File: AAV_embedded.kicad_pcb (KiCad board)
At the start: 4 copper layers, 165.8 x 114.2 mm, 51 parts, among them J1 JTAG_SWD_CONN, J10 DRV_HIGH_C2, J11 DRV_LOW_C2, J12 DRV_HIGH_C3, J13 DRV_LOW_C3, J14 DRV_LOW_C1, J2 12v in, J3 USB_C_Receptacle_USB2.0_14P, J5 THR_EN_JMP, J6 GPIO_INTERNAL_PINS, J7 GPIO_EXT_PINS, J8 Conn_01x03_Pin, J9 DRV_HIGH_C1, SW1 DAC_ADDR, SW2 IO_EXT_ADDR, SW3 SW_DIP_x03, SW4 5v_USB_EN, SW5 DAC_EN, U1 DAC101C081CIMK, U2 PCA9555D, U3 LD1117S50TR_SOT223, U4 LD1117S33TR_SOT223, U5 FXMA108

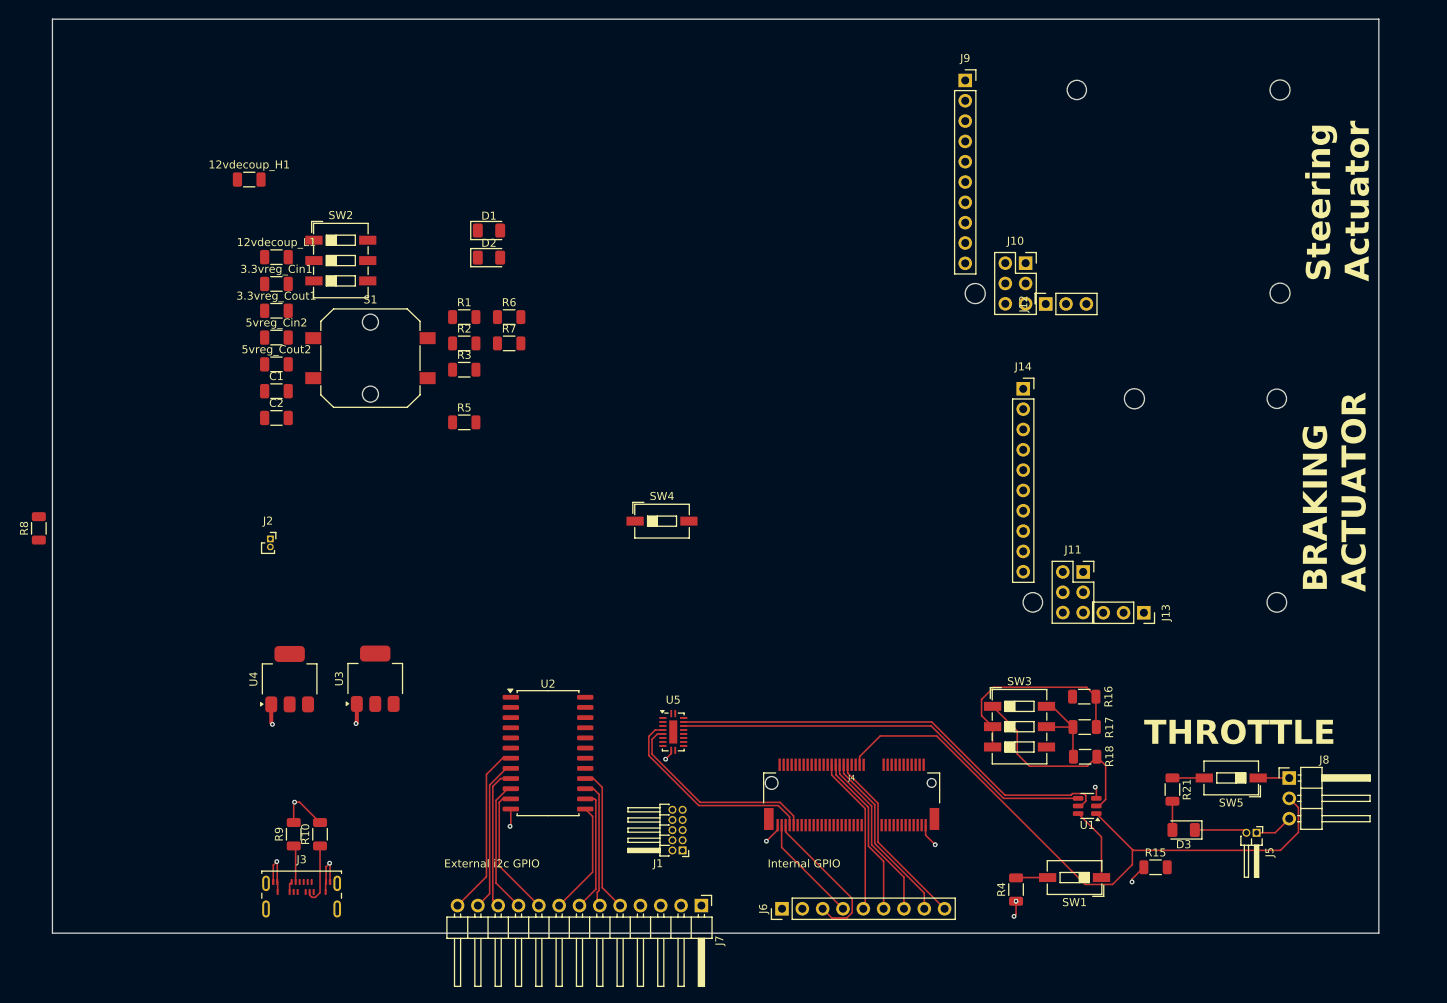
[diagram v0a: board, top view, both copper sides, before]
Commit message: board layout v1
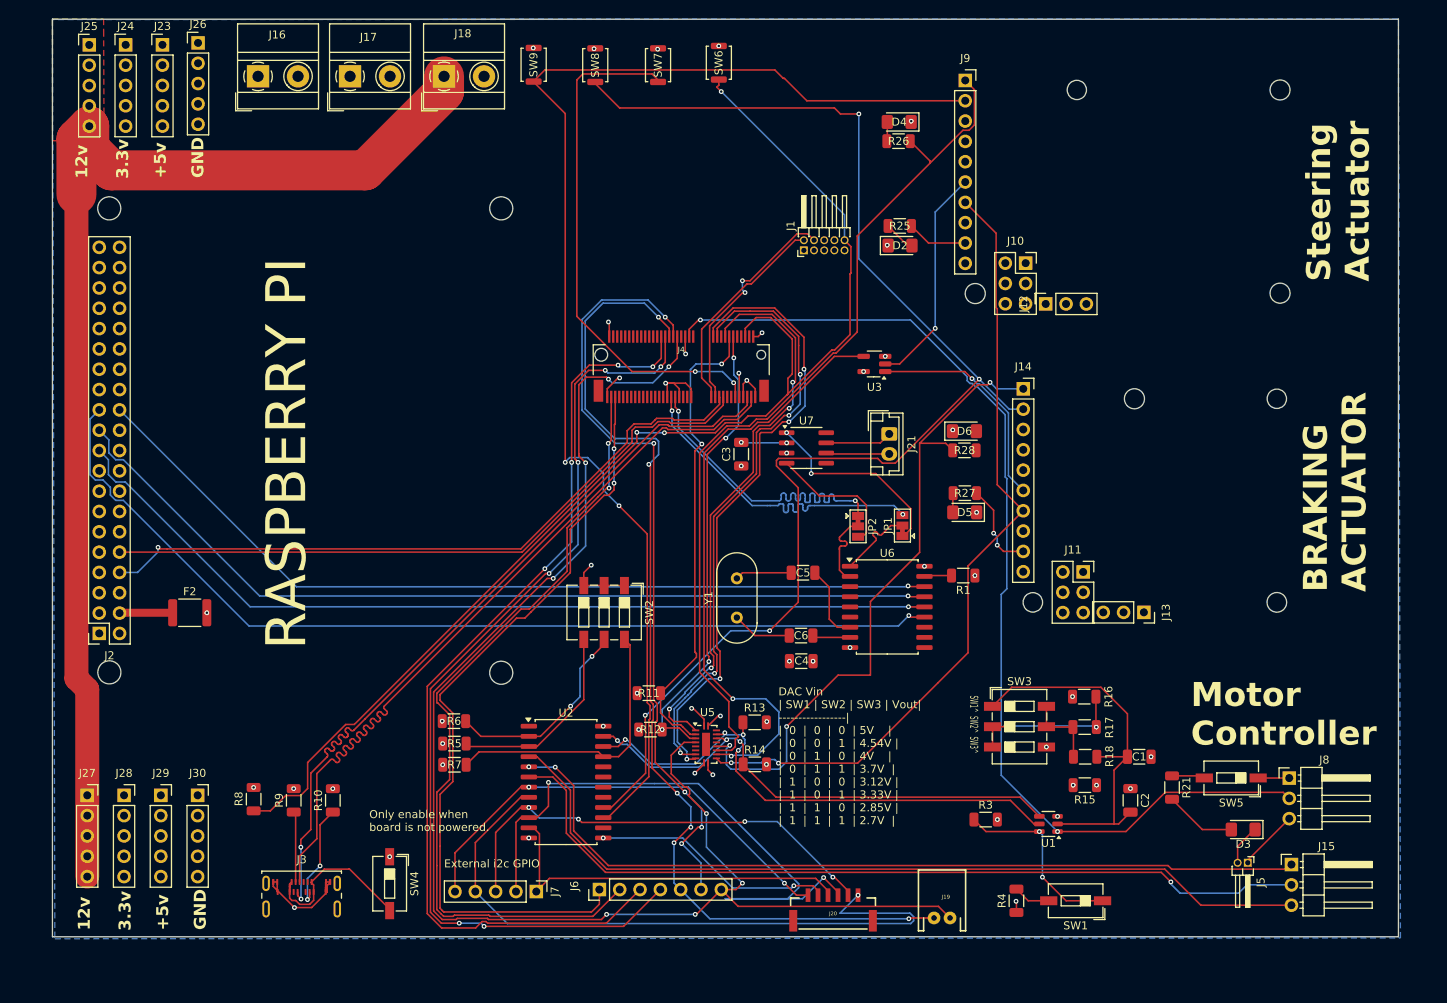
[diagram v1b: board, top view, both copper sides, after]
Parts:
- removed 12vdecoup_H1: 0.1uF, Capacitor_SMD:C_1206_3216Metric
- removed 12vdecoup_L1: 100uF, Capacitor_SMD:C_1206_3216Metric
- removed 3.3vreg_Cin1, 5vreg_Cin2: 100nF, Capacitor_SMD:C_1206_3216Metric
- removed 3.3vreg_Cout1, 5vreg_Cout2: 10uF, Capacitor_SMD:C_1206_3216Metric
- removed D1: D_Schottky_low_forward, Diode_SMD:D_1206_3216Metric
- removed R2: 2k, Resistor_SMD:R_1206_3216Metric
- removed S1: GPTS203211B, Button_Switch_SMD:SW_Push_1P1T_NO_CK_PTS125Sx43PSMTR
- removed U4: LD1117S33TR_SOT223, Package_TO_SOT_SMD:SOT-223-3_TabPin2
- added C3: 0.1uF, Capacitor_SMD:C_1206_3216Metric, F.Cu at (134.1, 97.5)
- added C4: 0.1uF, Capacitor_SMD:C_1206_3216Metric, F.Cu at (141.6, 123.4)
- added C5: 22pF, Capacitor_SMD:C_1206_3216Metric, F.Cu at (141.8, 112.3)
- added C6: 22pF, Capacitor_SMD:C_1206_3216Metric, F.Cu at (141.5, 120.2)
- added D4: LED, LED_SMD:LED_1206_3216Metric_Pad1.42x1.75mm_HandSolder, F.Cu at (153.8, 56.0)
- added D5: LED, LED_SMD:LED_1206_3216Metric_Pad1.42x1.75mm_HandSolder, F.Cu at (162.0, 104.8)
- added D6: LED, LED_SMD:LED_1206_3216Metric_Pad1.42x1.75mm_HandSolder, F.Cu at (161.9, 94.7)
- added F2: Polyfuse_3A_15V, Fuse:Fuse_1812_4532Metric, F.Cu at (65.1, 117.3)
- added J15: Brake/FwRev, Connector_PinHeader_2.54mm:PinHeader_1x03_P2.54mm_Horizontal, F.Cu at (202.8, 148.8)
- added J16: 5v_in, TerminalBlock_MetzConnect:TerminalBlock_MetzConnect_Type011_RT05502HBWC_1x02_P5.00mm_Horizontal, F.Cu at (73.7, 50.3)
- added J17: 3.3v_in, TerminalBlock_MetzConnect:TerminalBlock_MetzConnect_Type011_RT05502HBWC_1x02_P5.00mm_Horizontal, F.Cu at (85.2, 50.3)
- added J18: 12v_in, TerminalBlock_MetzConnect:TerminalBlock_MetzConnect_Type011_RT05502HBWC_1x02_P5.00mm_Horizontal, F.Cu at (96.9, 50.3)
- added J19: ~, SparkFun-Connectors:JST-2-PTH, F.Cu at (159.2, 155.5)
- added J20: ~, SparkFun-Connectors:JST-6-SMD-1.25MM-LOCKING, F.Cu at (145.5, 155.9)
- added J21: CAN, Connector_JST:JST_EH_B2B-EH-A_1x02_P2.50mm_Vertical, F.Cu at (152.6, 95.0)
- added J23: 5v_rail, Connector_PinHeader_2.54mm:PinHeader_1x05_P2.54mm_Vertical, F.Cu at (61.7, 46.4)
- added J24: 3.3v_rail, Connector_PinHeader_2.54mm:PinHeader_1x05_P2.54mm_Vertical, F.Cu at (57.1, 46.4)
- added J25: 12v_rail, Connector_PinHeader_2.54mm:PinHeader_1x05_P2.54mm_Vertical, F.Cu at (52.5, 46.4)
- added J26: GND_rail, Connector_PinHeader_2.54mm:PinHeader_1x05_P2.54mm_Vertical, F.Cu at (66.2, 46.1)
- added J27: 12v_rail_f, Connector_PinSocket_2.54mm:PinSocket_1x05_P2.54mm_Vertical, F.Cu at (52.3, 140.2)
- added J28: 3.3v_rail_f, Connector_PinSocket_2.54mm:PinSocket_1x05_P2.54mm_Vertical, F.Cu at (56.9, 140.2)
- added J29: 5v_rail_f, Connector_PinSocket_2.54mm:PinSocket_1x05_P2.54mm_Vertical, F.Cu at (61.5, 140.2)
- added J30: GND_rail_f, Connector_PinSocket_2.54mm:PinSocket_1x05_P2.54mm_Vertical, F.Cu at (66.1, 140.2)
- added JP1: CAN_TXD_SEL, Jumper:SolderJumper-3_P1.3mm_Bridged12_Pad1.0x1.5mm, F.Cu at (154.2, 106.5)
- added JP2: CAN_RXD_SEL, Jumper:SolderJumper-3_P1.3mm_Bridged12_Pad1.0x1.5mm, F.Cu at (148.7, 106.5)
- added R11: 2k, Resistor_SMD:R_1206_3216Metric, F.Cu at (122.5, 127.4)
- added R12: 2k, Resistor_SMD:R_1206_3216Metric, F.Cu at (122.7, 131.9)
- added R13: 2k, Resistor_SMD:R_1206_3216Metric, F.Cu at (135.7, 131.1)
- added R14: 2k, Resistor_SMD:R_1206_3216Metric, F.Cu at (135.8, 136.3)
- added R25: 10k, Resistor_SMD:R_1206_3216Metric, F.Cu at (153.9, 69.0)
- added R26: 10k, Resistor_SMD:R_1206_3216Metric, F.Cu at (153.7, 58.4)
- added R27: 10k, Resistor_SMD:R_1206_3216Metric, F.Cu at (162.0, 102.4)
- added R28: 10k, Resistor_SMD:R_1206_3216Metric, F.Cu at (161.9, 97.0)
- added SW6: ~{RESET_uMOD}, Button_Switch_SMD:SW_Push_SPST_NO_Alps_SKRK, F.Cu at (131.2, 48.6)
- added SW7: ~{BOOT_uMOD}, Button_Switch_SMD:SW_Push_SPST_NO_Alps_SKRK, F.Cu at (123.7, 48.9)
- added SW8: ~{RESET_BRK}, Button_Switch_SMD:SW_Push_SPST_NO_Alps_SKRK, F.Cu at (115.8, 48.9)
- added SW9: ~{RESET_STR}, Button_Switch_SMD:SW_Push_SPST_NO_Alps_SKRK, F.Cu at (108.1, 48.9)
- added U6: MCP2515-xSO, Package_SO:SOIC-18W_7.5x11.6mm_P1.27mm, F.Cu at (152.3, 116.6)
- added U7: SN65HVD230, Package_SO:SOIC-8_3.9x4.9mm_P1.27mm, F.Cu at (142.2, 96.8)
- added Y1: 16MHz, Crystal:Crystal_HC18-U_Vertical, F.Cu at (133.5, 118.0)
- D2: value D_TVS -> LED; footprint Diode_SMD:D_1206_3216Metric -> LED_SMD:LED_1206_3216Metric_Pad1.42x1.75mm_HandSolder
- D3: footprint LED_SMD:LED_1206_3216Metric -> LED_SMD:LED_1206_3216Metric_Pad1.42x1.75mm_HandSolder
- J2: value 12v in -> Raspberry_Pi_4; footprint Connector_PinSocket_1.00mm:PinSocket_1x02_P1.00mm_Vertical -> Connector_PinSocket_2.54mm:PinSocket_2x20_P2.54mm_Vertical
- J6: value GPIO_INTERNAL_PINS -> Conn_01x07; footprint Connector_PinHeader_2.54mm:PinHeader_1x09_P2.54mm_Vertical -> Connector_PinHeader_2.54mm:PinHeader_1x07_P2.54mm_Vertical
- J7: value GPIO_EXT_PINS -> Conn_01x05; footprint Connector_PinHeader_2.54mm:PinHeader_1x13_P2.54mm_Horizontal -> Connector_PinHeader_2.54mm:PinHeader_1x05_P2.54mm_Vertical
- J8: value Conn_01x03_Pin -> Throttle Connector
- R1: value 2k -> 10k
- SW5: value DAC_EN -> THR_EN
- U3: value LD1117S50TR_SOT223 -> 74AHC1G08; footprint Package_TO_SOT_SMD:SOT-223-3_TabPin2 -> Package_TO_SOT_SMD:SOT-23-5_HandSoldering
- moved C1 117.1 mm to (183.8, 135.3), turned to 180 degrees
- moved C2 117.0 mm to (182.7, 140.8), turned to -90 degrees
- moved R3 86.1 mm to (164.6, 143.2)
- moved J1 76.5 mm to (141.9, 72.0), turned to 90 degrees
- moved U3 73.8 mm to (150.7, 86.2), turned to 180 degrees
- moved R1 70.2 mm to (161.8, 112.7), turned to 180 degrees
- moved J4 57.6 mm to (126.5, 85.1)
- moved SW4 56.7 mm to (90.1, 151.2), turned to -90 degrees
- moved SW2 54.9 mm to (116.9, 117.3), turned to -90 degrees
- moved R7 53.1 mm to (98.2, 136.3)
- moved D2 51.4 mm to (153.9, 71.5)
- moved R6 51.0 mm to (98.1, 130.9)
- moved R8 43.2 mm to (73.1, 140.7), turned to -90 degrees
- moved R5 40.2 mm to (98.2, 133.7)
- moved J2 24.4 mm to (53.8, 119.9), turned to 180 degrees
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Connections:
- net RST renamed ~{RESET_uMOD}
- D2 pad 1: Net-(D1-A) -> GND
- D2 pad 2: GND -> Net-(D2-A)
- J14 pad 1: ERR_LOW -> ERR_BRK
- J14 pad 2: ~{RST_LOW} -> ~{RST_BRK}
- J14 pad 6: TX_LOW_5v -> TX_BRK_5v
- J14 pad 7: RX_LOW_5v -> RX_DRV_5v
- J14 pad 9: 5v_reg_LOW -> 5v_reg_BRK
- J2 pad 1: GND -> Net-(J2-3V3-Pad1)
- J2 pad 2: Net-(D1-A) -> Net-(F2-Pad1)
- J4 pad 11: unconnected-(J4-~{BOOT}-Pad11) -> ~{BOOT_uMOD}
- J4 pad 17: unconnected-(J4-TX1-Pad17) -> uMod_TX1
- J4 pad 19: unconnected-(J4-RX1-Pad19) -> uMod_RX1
- J4 pad 2: Net-(J4-3.3V-Pad2) -> +3.3V
- J4 pad 20: unconnected-(J4-RX2-Pad20) -> TX_DRV_L
- J4 pad 22: unconnected-(J4-TX2-Pad22) -> RX_DRV_L
- J4 pad 40: GPIO_INTERNAL_0 -> ~{E-STOP}
- J4 pad 41: unconnected-(J4-CAN-RX-Pad41) -> CAN_RXD
- J4 pad 42: GPIO_INTERNAL_1 -> ERR_L
- J4 pad 43: unconnected-(J4-CAN-TX-Pad43) -> CAN_TXD
- J4 pad 44: GPIO_INTERNAL_2 -> ~{E-STOP-TRIG}
- J4 pad 51: SDA _MCTRL_L -> unconnected-(J4-I2C_SDA1-Pad51)
- J4 pad 53: SCL_MCTRL_L -> unconnected-(J4-I2C_SCL1-Pad53)
- J4 pad 67: ERR_HIGH_L -> GPIO_INTERNAL_8
- J4 pad 69: ERR_LOW_L -> GPIO_INTERNAL_7
- J4 pad 74: Net-(J4-3.3V-Pad2) -> +3.3V
- J4 pad 9: unconnected-(J4-USB_VIN-Pad9) -> +5V
- J6 pad 1: GPIO_INTERNAL_8 -> GPIO_INTERNAL_6
- J6 pad 2: GPIO_INTERNAL_7 -> GPIO_INTERNAL_5
- J6 pad 3: GPIO_INTERNAL_6 -> GPIO_INTERNAL_4
- J6 pad 4: GPIO_INTERNAL_5 -> GPIO_INTERNAL_3
- J6 pad 5: GPIO_INTERNAL_4 -> ~{E-STOP-TRIG}
- J6 pad 6: GPIO_INTERNAL_3 -> ERR_L
- J6 pad 7: GPIO_INTERNAL_2 -> ~{E-STOP}
- J7 pad 1: GPIO_EXT_12 -> GPIO_EXT_4
- J7 pad 2: GPIO_EXT_11 -> GPIO_EXT_3
- J7 pad 3: GPIO_EXT_10 -> GPIO_EXT_2
- J7 pad 4: GPIO_EXT_9 -> GPIO_EXT_1
- J7 pad 5: GPIO_EXT_8 -> GPIO_EXT_0
- J9 pad 1: ERR_HIGH -> ERR_STR
- J9 pad 2: ~{RST_HIGH} -> ~{RST_STR}
- J9 pad 6: TX_HIGH_5v -> TX_STR_5v
- J9 pad 7: RX_HIGH_5v -> RX_DRV_5v
- J9 pad 9: 5v_reg_HIGH -> 5v_reg_STR
- R1 pad 1: +5V -> GND
- R1 pad 2: SCL_1_H -> Net-(U6-~{RESET})
- U2 pad 15: GPIO_EXT_7 -> ~{RST_STR}
- U2 pad 16: GPIO_EXT_8 -> ~{RST_BRK}
- U3 pad 1: GND -> TX_BRK_5v
- U3 pad 2: +5V -> TX_STR_5v
- U3 pad 3: +12v -> GND
- U5 pad 12: unconnected-(U5-B7-Pad12) -> RX_DRV_5v
- U5 pad 13: unconnected-(U5-B6-Pad13) -> TX_DRV_5v
- U5 pad 14: unconnected-(U5-B5-Pad14) -> ERR_STR
- U5 pad 15: ERR_HIGH -> ERR_BRK
- U5 pad 16: ERR_LOW -> ~{ERR}
- U5 pad 5: ERR_LOW_L -> ~{E-STOP}
- U5 pad 6: ERR_HIGH_L -> ERR_BRK_L
- U5 pad 7: unconnected-(U5-A5-Pad7) -> ERR_STR_L
- U5 pad 8: unconnected-(U5-A6-Pad8) -> TX_DRV_L
- U5 pad 9: unconnected-(U5-A7-Pad9) -> RX_DRV_L
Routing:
- net ~{E-STOP}: track 0.00 -> 186.2 mm, vias 0 -> 8
- net ~{RST_BRK}: track 0.00 -> 169.4 mm, vias 0 -> 4
- net ~{RST_STR}: track 0.00 -> 159.5 mm, vias 0 -> 2
- net ~{RESET_uMOD}: track 0.00 -> 156.7 mm, vias 0 -> 3
- net +12V: track 0.00 -> 150.5 mm
- net ~{E-STOP-TRIG}: track 0.00 -> 129.0 mm, vias 0 -> 6
- net CAN_SCK: track 0.00 -> 121.9 mm, vias 0 -> 1
- net CAN_MISO: track 0.00 -> 112.7 mm, vias 0 -> 1
- net CAN_MOSI: track 0.00 -> 112.3 mm, vias 0 -> 1
- net CAN_CS: track 0.00 -> 109.8 mm, vias 0 -> 1
- net ERR_STR: track 0.00 -> 109.6 mm
- net Fw/Rv: track 0.00 -> 106.1 mm
- net Brk_low: track 0.00 -> 105.0 mm, vias 0 -> 1
- net Brk_hi: track 0.00 -> 104.2 mm, vias 0 -> 2
- net GPIO_INTERNAL_3: track 20.5 -> 121.4 mm, vias 0 -> 6
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- added copper zone on F.Cu, net +12V
- added copper zone on B.Cu, net +3.3V
- added copper zone on In2.Cu, net +5V
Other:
- board size 165.8 x 114.2 mm -> 168.2 x 114.7 mm
- board text added: "+5v"
- board text added: "12v"
- board text added: "3.3v"
- board text added: "DAC Vin | SW1 | SW2 | SW3 | Vout| -----------------| | 0 | 0 | 0 | 5V | | 0 | 0 | 1 | 4.54V | | 0 | 1 | 0 | 4V | | 0 | 1 | 1 | 3.7V | | 1 | 0 | 0 | 3.12V | | 1 | 0 | 1 | 3.33V | | 1 | 1 | 0 | 2.85V | | 1 | 1 | 1 | 2.7V |"
- board text added: "GND"
- board text added: "Motor Controller"
- board text added: "Only enable when board is not powered."
- board text added: "RASPBERRY PI"
- board text added: "SW1^ SW2^ SW3^"
- board text removed: "Internal GPIO"
- board text removed: "THROTTLE"
